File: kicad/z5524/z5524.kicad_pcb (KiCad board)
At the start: 4 copper layers, 80 x 80 mm, 21 parts, among them J1 Conn_01x01, J2 Conn_01x02, J3 Conn_02x20_Odd_Even, U13 LM4040AIM3-2.5, U14 AD5328, U15 M24C02-WMN, U7 PCA9555D

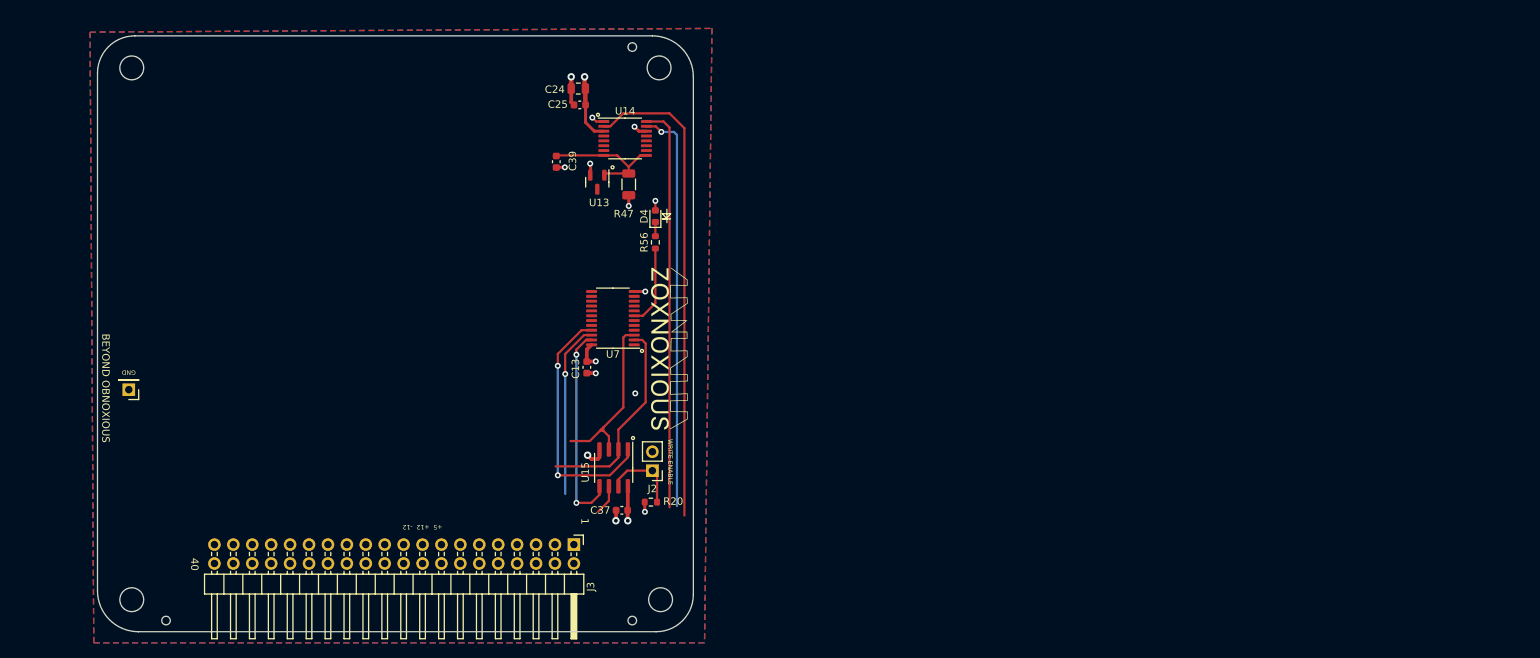
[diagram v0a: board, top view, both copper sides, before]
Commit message: schematic drafted- still needs some updates
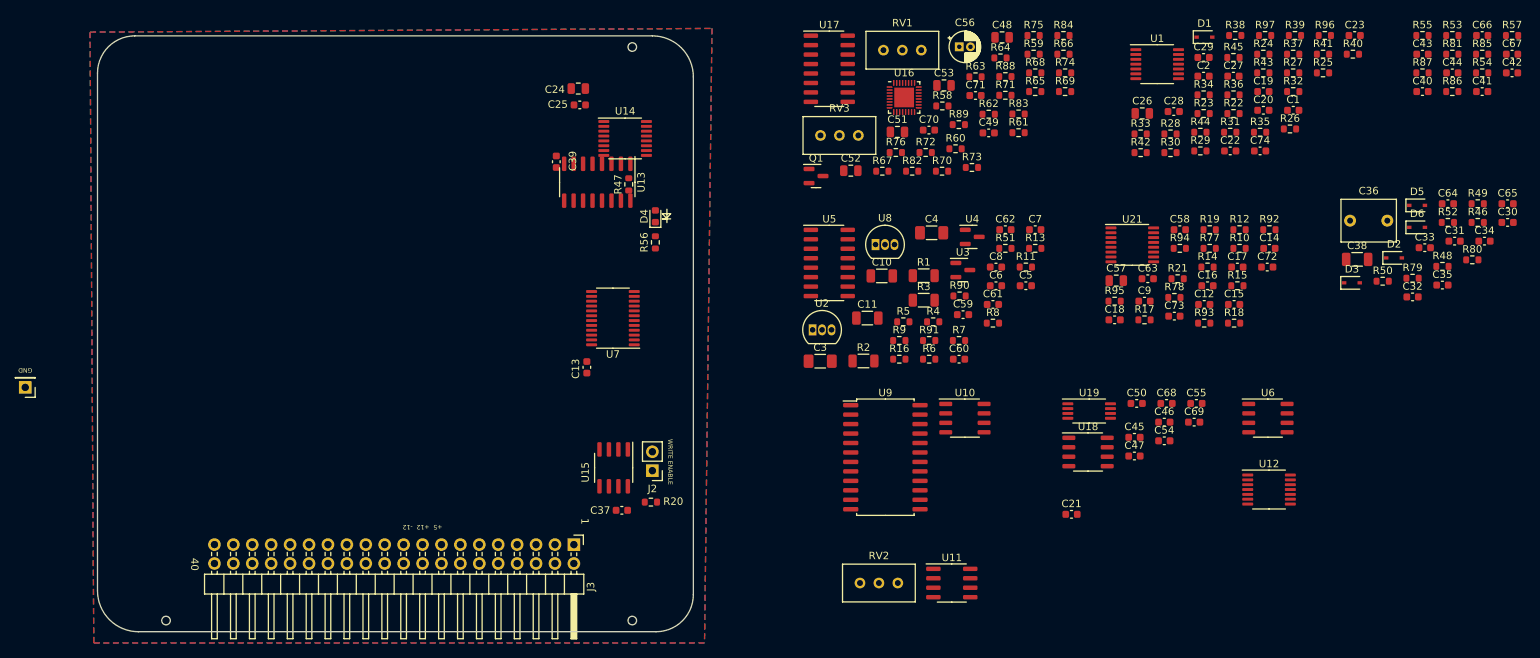
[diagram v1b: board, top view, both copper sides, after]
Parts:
- removed G***: LOGO, project_footprints:zoxnoxious_small
- removed H1, H2, H3, H4: MountingHole, MountingHole:MountingHole_3.2mm_M3
- added C1: 0.1u, Capacitor_SMD:C_0603_1608Metric, F.Cu at (225.9, 34.9)
- added C10: 1u, Capacitor_SMD:C_1206_3216Metric, F.Cu at (170.7, 57.1)
- added C11: 1u, Capacitor_SMD:C_1206_3216Metric, F.Cu at (168.8, 62.8)
- added C12: 10n, Capacitor_SMD:C_0603_1608Metric, F.Cu at (214.0, 61.0)
- added C14: 1u, Capacitor_SMD:C_0603_1608Metric, F.Cu at (222.7, 53.4)
- added C15: 1u, Capacitor_SMD:C_0603_1608Metric, F.Cu at (218.0, 61.0)
- added C16: 1u, Capacitor_SMD:C_0603_1608Metric, F.Cu at (214.4, 58.5)
- added C17: 0.1u, Capacitor_SMD:C_0603_1608Metric, F.Cu at (218.4, 55.9)
- added C18: 0.1u, Capacitor_SMD:C_0603_1608Metric, F.Cu at (202.0, 63.0)
- added C19: 22n, Capacitor_SMD:C_0603_1608Metric, F.Cu at (221.9, 32.4)
- added C2: 0.1u, Capacitor_SMD:C_0603_1608Metric, F.Cu at (213.9, 30.3)
- added C20: 2u2, Capacitor_SMD:C_0603_1608Metric, F.Cu at (221.9, 34.9)
- added C21: 2u2, Capacitor_SMD:C_0603_1608Metric, F.Cu at (196.2, 89.1)
- added C22: 15n, Capacitor_SMD:C_0603_1608Metric, F.Cu at (217.5, 40.4)
- added C23: 1n, Capacitor_SMD:C_0603_1608Metric, F.Cu at (234.2, 24.9)
- added C26: 47n, Capacitor_SMD:C_0805_2012Metric, F.Cu at (205.7, 35.3)
- added C27: 22n, Capacitor_SMD:C_0603_1608Metric, F.Cu at (217.9, 30.3)
- added C28: 22n, Capacitor_SMD:C_0603_1608Metric, F.Cu at (209.9, 35.1)
- added C29: 22n, Capacitor_SMD:C_0603_1608Metric, F.Cu at (213.9, 27.8)
- added C3: 1u, Capacitor_SMD:C_1206_3216Metric_Pad1.33x1.80mm_HandSolder, F.Cu at (162.4, 68.6)
- added C30: 0.1u, Capacitor_SMD:C_0603_1608Metric, F.Cu at (254.7, 50.0)
- added C31: 0.1u, Capacitor_SMD:C_0603_1608Metric, F.Cu at (247.6, 52.5)
- added C32: 560pF, Capacitor_SMD:C_0603_1608Metric, F.Cu at (242.0, 60.0)
- added C33: 33nF, Capacitor_SMD:C_0603_1608Metric, F.Cu at (243.6, 53.3)
- added C34: 33nF, Capacitor_SMD:C_0603_1608Metric, F.Cu at (251.6, 52.5)
- added C35: 33nF, Capacitor_SMD:C_0603_1608Metric, F.Cu at (246.0, 58.4)
- added C36: 4.7u, Capacitor_THT:C_Rect_L7.2mm_W5.5mm_P5.00mm_FKS2_FKP2_MKS2_MKP2, F.Cu at (233.6, 49.7)
- added C38: 2n, Capacitor_SMD:C_1206_3216Metric, F.Cu at (234.5, 54.9)
- added C4: 1u, Capacitor_SMD:C_1206_3216Metric_Pad1.33x1.80mm_HandSolder, F.Cu at (177.4, 51.3)
- added C40: 0.1u, Capacitor_SMD:C_0603_1608Metric, F.Cu at (243.3, 32.4)
- added C41: 0.1u, Capacitor_SMD:C_0603_1608Metric, F.Cu at (251.3, 32.4)
- added C42: 0.1u, Capacitor_SMD:C_0603_1608Metric, F.Cu at (255.3, 29.9)
- added C43: 33p, Capacitor_SMD:C_0603_1608Metric, F.Cu at (243.3, 27.4)
- added C44: 33p, Capacitor_SMD:C_0603_1608Metric, F.Cu at (247.3, 29.9)
- added C45: 0.1u, Capacitor_SMD:C_0603_1608Metric, F.Cu at (204.6, 78.8)
- added C46: 0.1u, Capacitor_SMD:C_0603_1608Metric, F.Cu at (208.6, 76.8)
- added C47: 0.1u, Capacitor_SMD:C_0603_1608Metric, F.Cu at (204.6, 81.3)
- added C48: 10u, Capacitor_SMD:C_0805_2012Metric, F.Cu at (186.8, 25.1)
- added C49: 3.9n, Capacitor_SMD:C_0603_1608Metric, F.Cu at (185.1, 37.9)
- added C5: 0.1u, Capacitor_SMD:C_0603_1608Metric, F.Cu at (190.0, 58.5)
- added C50: 0.1u, Capacitor_SMD:C_0603_1608Metric, F.Cu at (204.9, 74.2)
- added C51: 100p, Capacitor_SMD:C_0805_2012Metric, F.Cu at (172.8, 37.8)
- added C52: 100p, Capacitor_SMD:C_0805_2012Metric, F.Cu at (166.5, 43.0)
- added C53: 100p, Capacitor_SMD:C_0805_2012Metric, F.Cu at (179.1, 31.6)
- added C54: 0.1u, Capacitor_SMD:C_0603_1608Metric, F.Cu at (208.6, 79.3)
- added C55: 0.1u, Capacitor_SMD:C_0603_1608Metric, F.Cu at (212.9, 74.2)
- added C56: 4u7, Capacitor_THT:CP_Radial_D4.0mm_P1.50mm, F.Cu at (181.1, 26.4)
- added C57: 4.7u, Capacitor_SMD:C_0805_2012Metric, F.Cu at (202.2, 57.8)
- added C58: 0.1u, Capacitor_SMD:C_0603_1608Metric, F.Cu at (210.7, 50.9)
- added C59: 100p, Capacitor_SMD:C_0603_1608Metric, F.Cu at (181.6, 62.3)
- added C6: 0.1u, Capacitor_SMD:C_0603_1608Metric, F.Cu at (186.0, 58.5)
- added C60: 0.1u, Capacitor_SMD:C_0603_1608Metric, F.Cu at (181.1, 68.3)
- added C61: 0.1u, Capacitor_SMD:C_0603_1608Metric, F.Cu at (185.6, 61.0)
- added C62: 100p, Capacitor_SMD:C_0603_1608Metric, F.Cu at (187.3, 50.9)
- added C63: 22n, Capacitor_SMD:C_0603_1608Metric, F.Cu at (206.4, 57.5)
- added C64: 0.1u, Capacitor_SMD:C_0603_1608Metric, F.Cu at (246.7, 47.4)
- added C65: 0.1u, Capacitor_SMD:C_0603_1608Metric, F.Cu at (254.7, 47.4)
- added C66: 5n, Capacitor_SMD:C_0603_1608Metric, F.Cu at (251.3, 24.9)
- added C67: 33p, Capacitor_SMD:C_0603_1608Metric, F.Cu at (255.3, 27.4)
- added C68: 0.1u, Capacitor_SMD:C_0603_1608Metric, F.Cu at (208.9, 74.2)
- added C69: 0.1u, Capacitor_SMD:C_0603_1608Metric, F.Cu at (212.6, 76.8)
- added C7: 0.1u, Capacitor_SMD:C_0603_1608Metric, F.Cu at (191.3, 50.9)
- added C70: 10n, Capacitor_SMD:C_0603_1608Metric, F.Cu at (177.0, 37.5)
- added C71: 10n, Capacitor_SMD:C_0603_1608Metric, F.Cu at (183.3, 32.9)
- added C72: 6.8n, Capacitor_SMD:C_0603_1608Metric, F.Cu at (222.4, 55.9)
- added C73: 6.8n, Capacitor_SMD:C_0603_1608Metric, F.Cu at (210.0, 62.5)
- added C74: 22n, Capacitor_SMD:C_0603_1608Metric, F.Cu at (221.5, 40.4)
- added C8: 0.1u, Capacitor_SMD:C_0603_1608Metric, F.Cu at (186.0, 55.9)
- added C9: 22n, Capacitor_SMD:C_0603_1608Metric, F.Cu at (206.0, 60.5)
- added D1: 1N5819WS, Diode_SMD:D_SOD-323, F.Cu at (214.0, 25.1)
- added D2: 1N4148WS, Diode_SMD:D_SOD-323, F.Cu at (239.5, 54.7)
- added D3: 1N4148WS, Diode_SMD:D_SOD-323, F.Cu at (233.8, 58.1)
- added D5: 1N4148WS, Diode_SMD:D_SOD-323, F.Cu at (242.6, 47.7)
- added D6: 1N4148WS, Diode_SMD:D_SOD-323, F.Cu at (242.6, 50.6)
- added Q1: 2N7002K, Package_TO_SOT_SMD:SOT-23, F.Cu at (161.9, 43.7)
- added R1: 1k, Resistor_SMD:R_1206_3216Metric, F.Cu at (176.3, 57.1)
- added R10: 5k1, Resistor_SMD:R_0603_1608Metric, F.Cu at (218.7, 53.4)
- added R11: 20k, Resistor_SMD:R_0603_1608Metric, F.Cu at (190.0, 55.9)
- added R12: 10k, Resistor_SMD:R_0603_1608Metric, F.Cu at (218.7, 50.9)
- added R13: 10k, Resistor_SMD:R_0603_1608Metric, F.Cu at (191.3, 53.4)
- added R14: 22k, Resistor_SMD:R_0603_1608Metric, F.Cu at (214.4, 55.9)
- added R15: 22k, Resistor_SMD:R_0603_1608Metric, F.Cu at (218.4, 58.5)
- added R16: 20k, Resistor_SMD:R_0603_1608Metric, F.Cu at (173.1, 68.3)
- added R17: 10k, Resistor_SMD:R_0603_1608Metric, F.Cu at (206.0, 63.0)
- added R18: 110, Resistor_SMD:R_0603_1608Metric, F.Cu at (218.0, 63.5)
- added R19: 110, Resistor_SMD:R_0603_1608Metric, F.Cu at (214.7, 50.9)
- added R2: 240, Resistor_SMD:R_1206_3216Metric, F.Cu at (168.2, 68.5)
- added R21: 110, Resistor_SMD:R_0603_1608Metric, F.Cu at (210.4, 57.5)
- added R22: 5k1, Resistor_SMD:R_0603_1608Metric, F.Cu at (217.9, 35.3)
- added R23: 110k, Resistor_SMD:R_0603_1608Metric, F.Cu at (213.9, 35.3)
- added R24: 10k, Resistor_SMD:R_0603_1608Metric, F.Cu at (221.9, 27.4)
- added R25: 20k, Resistor_SMD:R_0603_1608Metric, F.Cu at (229.9, 29.9)
- added R26: 47k, Resistor_SMD:R_0603_1608Metric, F.Cu at (225.5, 37.4)
- added R27: 20k, Resistor_SMD:R_0603_1608Metric, F.Cu at (225.9, 29.9)
- added R28: 36k, Resistor_SMD:R_0603_1608Metric, F.Cu at (209.5, 38.1)
- added R29: 30k, Resistor_SMD:R_0603_1608Metric, F.Cu at (213.5, 40.4)
- added R3: ?, Resistor_SMD:R_1206_3216Metric, F.Cu at (176.3, 60.4)
- added R30: 39k, Resistor_SMD:R_0603_1608Metric, F.Cu at (209.5, 40.6)
- added R31: 10k, Resistor_SMD:R_0603_1608Metric, F.Cu at (217.5, 37.8)
- added R32: 15k, Resistor_SMD:R_0603_1608Metric, F.Cu at (225.9, 32.4)
- added R33: 51k, Resistor_SMD:R_0603_1608Metric, F.Cu at (205.4, 38.1)
- added R34: 47k, Resistor_SMD:R_0603_1608Metric, F.Cu at (213.9, 32.8)
- added R35: 11k, Resistor_SMD:R_0603_1608Metric, F.Cu at (221.5, 37.8)
- added R36: 5k1, Resistor_SMD:R_0603_1608Metric, F.Cu at (217.9, 32.8)
- added R37: 22k, Resistor_SMD:R_0603_1608Metric, F.Cu at (225.9, 27.4)
- added R38: 4k7, Resistor_SMD:R_0603_1608Metric, F.Cu at (218.2, 24.9)
- added R39: 4k7, Resistor_SMD:R_0603_1608Metric, F.Cu at (226.2, 24.9)
- added R4: R, Resistor_SMD:R_0603_1608Metric, F.Cu at (177.6, 63.3)
- added R40: 5k1, Resistor_SMD:R_0603_1608Metric, F.Cu at (233.9, 27.4)
- added R41: 5k1, Resistor_SMD:R_0603_1608Metric, F.Cu at (229.9, 27.4)
- added R42: 100k, Resistor_SMD:R_0603_1608Metric, F.Cu at (205.4, 40.6)
- added R43: 5k1, Resistor_SMD:R_0603_1608Metric, F.Cu at (221.9, 29.9)
- added R44: 1M, Resistor_SMD:R_0603_1608Metric, F.Cu at (213.5, 37.8)
- added R45: 47k, Resistor_SMD:R_0603_1608Metric, F.Cu at (217.9, 27.8)
- added R46: 68k, Resistor_SMD:R_0603_1608Metric, F.Cu at (250.7, 50.0)
- added R48: 240k, Resistor_SMD:R_0603_1608Metric, F.Cu at (246.0, 55.9)
- added R49: 500, Resistor_SMD:R_0603_1608Metric, F.Cu at (250.7, 47.4)
- added R5: ?, Resistor_SMD:R_0603_1608Metric, F.Cu at (173.6, 63.3)
- added R50: 1k, Resistor_SMD:R_0603_1608Metric, F.Cu at (237.9, 57.8)
- added R51: 20k, Resistor_SMD:R_0603_1608Metric, F.Cu at (187.3, 53.4)
- added R52: 62k, Resistor_SMD:R_0603_1608Metric, F.Cu at (246.7, 50.0)
- added R53: 47k, Resistor_SMD:R_0603_1608Metric, F.Cu at (247.3, 24.9)
- added R54: 47k, Resistor_SMD:R_0603_1608Metric, F.Cu at (251.3, 29.9)
- added R55: 47k, Resistor_SMD:R_0603_1608Metric, F.Cu at (243.3, 24.9)
- added R57: 47k, Resistor_SMD:R_0603_1608Metric, F.Cu at (255.3, 24.9)
- added R58: 4k3, Resistor_SMD:R_0603_1608Metric, F.Cu at (178.8, 34.3)
- added R59: 47k, Resistor_SMD:R_0603_1608Metric, F.Cu at (191.1, 27.4)
- added R6: 13k, Resistor_SMD:R_0603_1608Metric, F.Cu at (177.1, 68.3)
- added R60: 49.9k, Resistor_SMD:R_0603_1608Metric, F.Cu at (180.6, 40.1)
- added R61: 10k, Resistor_SMD:R_0603_1608Metric, F.Cu at (189.1, 37.9)
- added R62: 270k, Resistor_SMD:R_0603_1608Metric, F.Cu at (185.1, 35.4)
- added R63: 100k, Resistor_SMD:R_0603_1608Metric, F.Cu at (183.3, 30.4)
- added R64: 22k, Resistor_SMD:R_0603_1608Metric, F.Cu at (186.6, 27.9)
- added R65: 270, Resistor_SMD:R_0603_1608Metric, F.Cu at (191.3, 32.4)
- added R66: 20k, Resistor_SMD:R_0603_1608Metric, F.Cu at (195.1, 27.4)
- added R67: 20k, Resistor_SMD:R_0603_1608Metric, F.Cu at (170.8, 43.1)
- added R68: 20k, Resistor_SMD:R_0603_1608Metric, F.Cu at (191.3, 29.9)
- added R69: 20k, Resistor_SMD:R_0603_1608Metric, F.Cu at (195.3, 32.4)
- added R7: 3k, Resistor_SMD:R_0603_1608Metric, F.Cu at (181.1, 65.8)
- added R70: 20k, Resistor_SMD:R_0603_1608Metric, F.Cu at (178.8, 43.1)
- added R71: 20k, Resistor_SMD:R_0603_1608Metric, F.Cu at (187.3, 32.9)
- added R72: 100, Resistor_SMD:R_0603_1608Metric, F.Cu at (176.6, 40.6)
- added R73: 100k, Resistor_SMD:R_0603_1608Metric, F.Cu at (182.8, 42.6)
- added R74: 20k, Resistor_SMD:R_0603_1608Metric, F.Cu at (195.3, 29.9)
- added R75: 499k, Resistor_SMD:R_0603_1608Metric, F.Cu at (191.1, 24.9)
- added R76: 10k, Resistor_SMD:R_0603_1608Metric, F.Cu at (172.6, 40.6)
- added R77: 5k1, Resistor_SMD:R_0603_1608Metric, F.Cu at (214.7, 53.4)
- added R78: 22k, Resistor_SMD:R_0603_1608Metric, F.Cu at (210.0, 60.0)
- added R79: 1k, Resistor_SMD:R_0603_1608Metric, F.Cu at (242.0, 57.4)
- added R8: 6k8, Resistor_SMD:R_0603_1608Metric, F.Cu at (185.6, 63.5)
- added R80: 62k, Resistor_SMD:R_0603_1608Metric, F.Cu at (250.0, 55.0)
- added R81: 100, Resistor_SMD:R_0603_1608Metric, F.Cu at (247.3, 27.4)
- added R82: 4k7, Resistor_SMD:R_0603_1608Metric, F.Cu at (174.8, 43.1)
- added R83: 4k7, Resistor_SMD:R_0603_1608Metric, F.Cu at (189.1, 35.4)
- added R84: 4k7, Resistor_SMD:R_0603_1608Metric, F.Cu at (195.1, 24.9)
- added R85: 47k, Resistor_SMD:R_0603_1608Metric, F.Cu at (251.3, 27.4)
- added R86: 47k, Resistor_SMD:R_0603_1608Metric, F.Cu at (247.3, 32.4)
- added R87: 47k, Resistor_SMD:R_0603_1608Metric, F.Cu at (243.3, 29.9)
- added R88: 10k, Resistor_SMD:R_0603_1608Metric, F.Cu at (187.3, 30.4)
- added R89: 10k, Resistor_SMD:R_0603_1608Metric, F.Cu at (181.0, 36.8)
- added R9: 6k8, Resistor_SMD:R_0603_1608Metric, F.Cu at (173.1, 65.8)
- added R90: 1k, Resistor_SMD:R_0603_1608Metric, F.Cu at (181.1, 59.8)
- added R91: 1k, Resistor_SMD:R_0603_1608Metric, F.Cu at (177.1, 65.8)
- added R92: 18k, Resistor_SMD:R_0603_1608Metric, F.Cu at (222.7, 50.9)
- added R93: 18k, Resistor_SMD:R_0603_1608Metric, F.Cu at (214.0, 63.5)
- added R94: 82k, Resistor_SMD:R_0603_1608Metric, F.Cu at (210.7, 53.4)
- added R95: 82k, Resistor_SMD:R_0603_1608Metric, F.Cu at (202.0, 60.5)
- added R96: 10k, Resistor_SMD:R_0603_1608Metric, F.Cu at (230.2, 24.9)
- added R97: 10k, Resistor_SMD:R_0603_1608Metric, F.Cu at (222.2, 24.9)
- added RV1: 5k, Potentiometer_THT:Potentiometer_Bourns_3296W_Vertical, F.Cu at (176.0, 26.8)
- added RV2: 5k, Potentiometer_THT:Potentiometer_Bourns_3296W_Vertical, F.Cu at (172.8, 98.4)
- added RV3: 5k, Potentiometer_THT:Potentiometer_Bourns_3296W_Vertical, F.Cu at (167.6, 38.3)
- added U1: TL074, Package_SO:TSSOP-14_4.4x5mm_P0.65mm, F.Cu at (207.7, 28.7)
- added U10: TL072, Package_SO:SO-8_3.9x4.9mm_P1.27mm, F.Cu at (181.9, 76.2)
- added U11: NE5532, Package_SO:SOIC-8_3.9x4.9mm_P1.27mm, F.Cu at (180.1, 98.4)
- added U12: TL074, Package_SO:TSSOP-14_4.4x5mm_P0.65mm, F.Cu at (222.7, 85.8)
- added U16: SSI2130, Package_DFN_QFN:QFN-32-1EP_4x4mm_P0.4mm_EP2.65x2.65mm, F.Cu at (173.7, 33.2)
- added U17: DG442xY, Package_SO:SOIC-16_3.9x9.9mm_P1.27mm, F.Cu at (163.7, 29.3)
- added U18: TL072, Package_SO:SO-8_3.9x4.9mm_P1.27mm, F.Cu at (198.4, 80.8)
- added U19: LM311, Package_SO:TSSOP-8_4.4x3mm_P0.65mm, F.Cu at (198.5, 75.3)
- added U2: LM337L_TO92, Package_TO_SOT_THT:TO-92_Inline, F.Cu at (161.4, 64.4)
- added U21: AD5328, Package_SO:TSSOP-16_4.4x5mm_P0.65mm, F.Cu at (204.3, 53.0)
- added U3: LM4040BIM3-2.5, Package_TO_SOT_SMD:SOT-23, F.Cu at (181.6, 56.3)
- added U4: LM4040BIM3-4.1, Package_TO_SOT_SMD:SOT-23, F.Cu at (182.8, 51.9)
- added U5: DG442xY, Package_SO:SOIC-16_3.9x9.9mm_P1.27mm, F.Cu at (163.7, 55.4)
- added U6: TL072, Package_SO:SO-8_3.9x4.9mm_P1.27mm, F.Cu at (222.5, 76.2)
- added U8: LM78L05_TO92, Package_TO_SOT_THT:TO-92_Inline, F.Cu at (169.9, 52.9)
- added U9: AS3394, Package_SO:SOIC-24W_7.5x15.4mm_P1.27mm, F.Cu at (171.2, 81.5)
- R47: value 4k7 -> 1k; footprint Resistor_SMD:R_1206_3216Metric -> Resistor_SMD:R_0603_1608Metric
- U13: value LM4040AIM3-2.5 -> AS3364; footprint Package_TO_SOT_SMD:SOT-23 -> Package_SO:SOIC-16_3.9x9.9mm_P1.27mm
- moved J1 13.9 mm to (55.7, 72.1)
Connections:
- C39 pad 1: /DAC/VREF_2.5V -> +12V
- J3 pad 21: /CARD1_OUT1 -> unconnected-(J3-Pad21)
- J3 pad 22: /CARD1_OUT2 -> unconnected-(J3-Pad22)
- J3 pad 23: /CARD2_OUT1 -> unconnected-(J3-Pad23)
- J3 pad 25: /CARD2_OUT2 -> unconnected-(J3-Pad25)
- J3 pad 26: /CARD3_OUT1 -> unconnected-(J3-Pad26)
- J3 pad 27: /CARD3_OUT2 -> unconnected-(J3-Pad27)
- J3 pad 29: /CARD4_OUT1 -> unconnected-(J3-Pad29)
- J3 pad 3: /SPI_MISO -> unconnected-(J3-Pad3)
- J3 pad 30: /CARD4_OUT2 -> unconnected-(J3-Pad30)
- J3 pad 31: /CARD5_OUT1 -> unconnected-(J3-Pad31)
- J3 pad 33: /CARD5_OUT2 -> unconnected-(J3-Pad33)
- J3 pad 34: /CARD6_OUT1 -> unconnected-(J3-Pad34)
- J3 pad 35: /CARD6_OUT2 -> unconnected-(J3-Pad35)
- J3 pad 37: /CARD7_OUT1 -> unconnected-(J3-Pad37)
- R47 pad 1: +5V -> GND
- R47 pad 2: /DAC/VREF_2.5V -> /AS3394/3394_EXT_IN
- U13 pad 1: /DAC/VREF_2.5V -> Net-(R81-Pad2)
- U13 pad 2: GND -> Net-(R53-Pad2)
- U13 pad 3: (no net) -> /SSI2130_MOD_CV
- U14 pad 10: unconnected-(U14-Pad10) -> /DAC 3394/RES_DAC_CV
- U14 pad 11: unconnected-(U14-Pad11) -> /DAC 3394/MOD_AMT_DAC_CV
- U14 pad 12: unconnected-(U14-Pad12) -> /DAC 3394/FINAL_GAIN_DAC_CV
- U14 pad 13: unconnected-(U14-Pad13) -> /DAC 3394/SSI2130_MOD_DAC_CV
- U14 pad 2: /SPI_CS0 -> /SPI_CS1
- U14 pad 4: unconnected-(U14-Pad4) -> /DAC 3394/VCO_DAC_CV
- U14 pad 5: unconnected-(U14-Pad5) -> /DAC 3394/PWM_DAC_CV
- U14 pad 6: unconnected-(U14-Pad6) -> /DAC 3394/Mix_DAC_CV
- U14 pad 7: unconnected-(U14-Pad7) -> /DAC 3394/VCF_DAC_CV
- U14 pad 8: /DAC/VREF_2.5V -> /VREF_4.096
- U14 pad 9: /DAC/VREF_2.5V -> /VREF_4.096
- U7 pad 11: unconnected-(U7-Pad11) -> /LED_CTRL
- U7 pad 17: unconnected-(U7-Pad17) -> /SOFTSYNC_2130_CTRL
- U7 pad 18: unconnected-(U7-Pad18) -> /HARDSYNC_2130_CTRL
- U7 pad 19: unconnected-(U7-Pad19) -> /FM2130_MOD_CTRL
- U7 pad 20: unconnected-(U7-Pad20) -> /PWM2130_MOD_CTRL
- U7 pad 4: unconnected-(U7-Pad4) -> /VCO3394_EXP_MOD_CTRL
- U7 pad 5: unconnected-(U7-Pad5) -> /VCF3394_MOD_CTRL
- U7 pad 6: unconnected-(U7-Pad6) -> /PWM3394_MOD_CTRL
- U7 pad 7: /LED_CTRL -> /WAVESELECT_MOD_CTRL
- U7 pad 8: unconnected-(U7-Pad8) -> /WAVESELECT_1
- U7 pad 9: unconnected-(U7-Pad9) -> /WAVESELECT_2
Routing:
- net /SPI_CS0: track 64.4 -> 0.00 mm
- net /SPI_CLK: track 54.4 -> 0.00 mm
- net /SPI_MOSI: track 54.4 -> 0.00 mm, vias 1 -> 0
- net /I2C_ADDR0: track 33.6 -> 0.00 mm, vias 2 -> 0
- net /SDA1: track 27.8 -> 0.00 mm, vias 2 -> 0
- net /I2C_ADDR1: track 27.5 -> 0.00 mm
- net /SCL1: track 27.4 -> 0.00 mm, vias 1 -> 0
- net /I2C_ADDR2: track 24.3 -> 0.00 mm
- net +5V: track 21.5 -> 0.00 mm, vias 6 -> 0
- net /DAC/VREF_2.5V: track 17.6 -> 0.00 mm
- net GND: track 114.9 -> 97.5 mm, vias 10 -> 0
- net /LED_CTRL: track 10.9 -> 0.00 mm
- net Net-(J2-Pad1): track 10.5 -> 0.00 mm
- net Net-(D4-Pad1): track 1.89 -> 0.00 mm
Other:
- board text removed: "BEYOND OBNOXIOUS"
